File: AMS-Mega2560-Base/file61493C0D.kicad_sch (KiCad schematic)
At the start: 50 parts, among them IC10 LM2597MX-ADJ_NOPB, IC11 LM2597M-3.3_NOPB, IC12 OPA2340PA, IC9 LM2670SX-5.0_NOPB, J21 Screw_Terminal_01x03, J22 Conn_01x07, Q21 IRF9Z34NPBF, Q22 IRF9610PBF-BE3, Q23 2N7000, Q5 2N7000, Q6 IRF9Z34NPBF, U1 BK_HTC-15M, U2 TL431LP

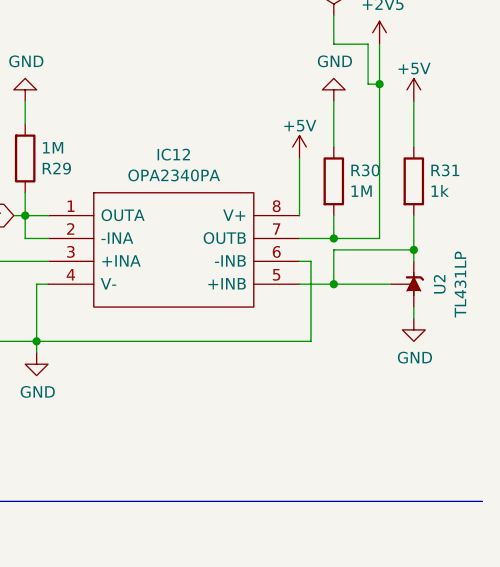
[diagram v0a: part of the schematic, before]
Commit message: still working on the fixes.
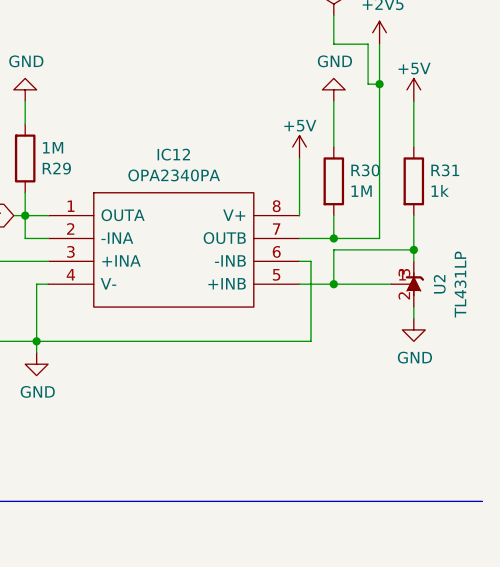
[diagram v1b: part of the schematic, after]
